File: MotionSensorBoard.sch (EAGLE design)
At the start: 21 parts, among them J1 PRGM, J2 POWER_JACKPTH, U1 ATTINY2313A-SUR, U2 ISO7221ADR, U4 NCP1117ST50T3G, U5 LM1117MPX-3.3

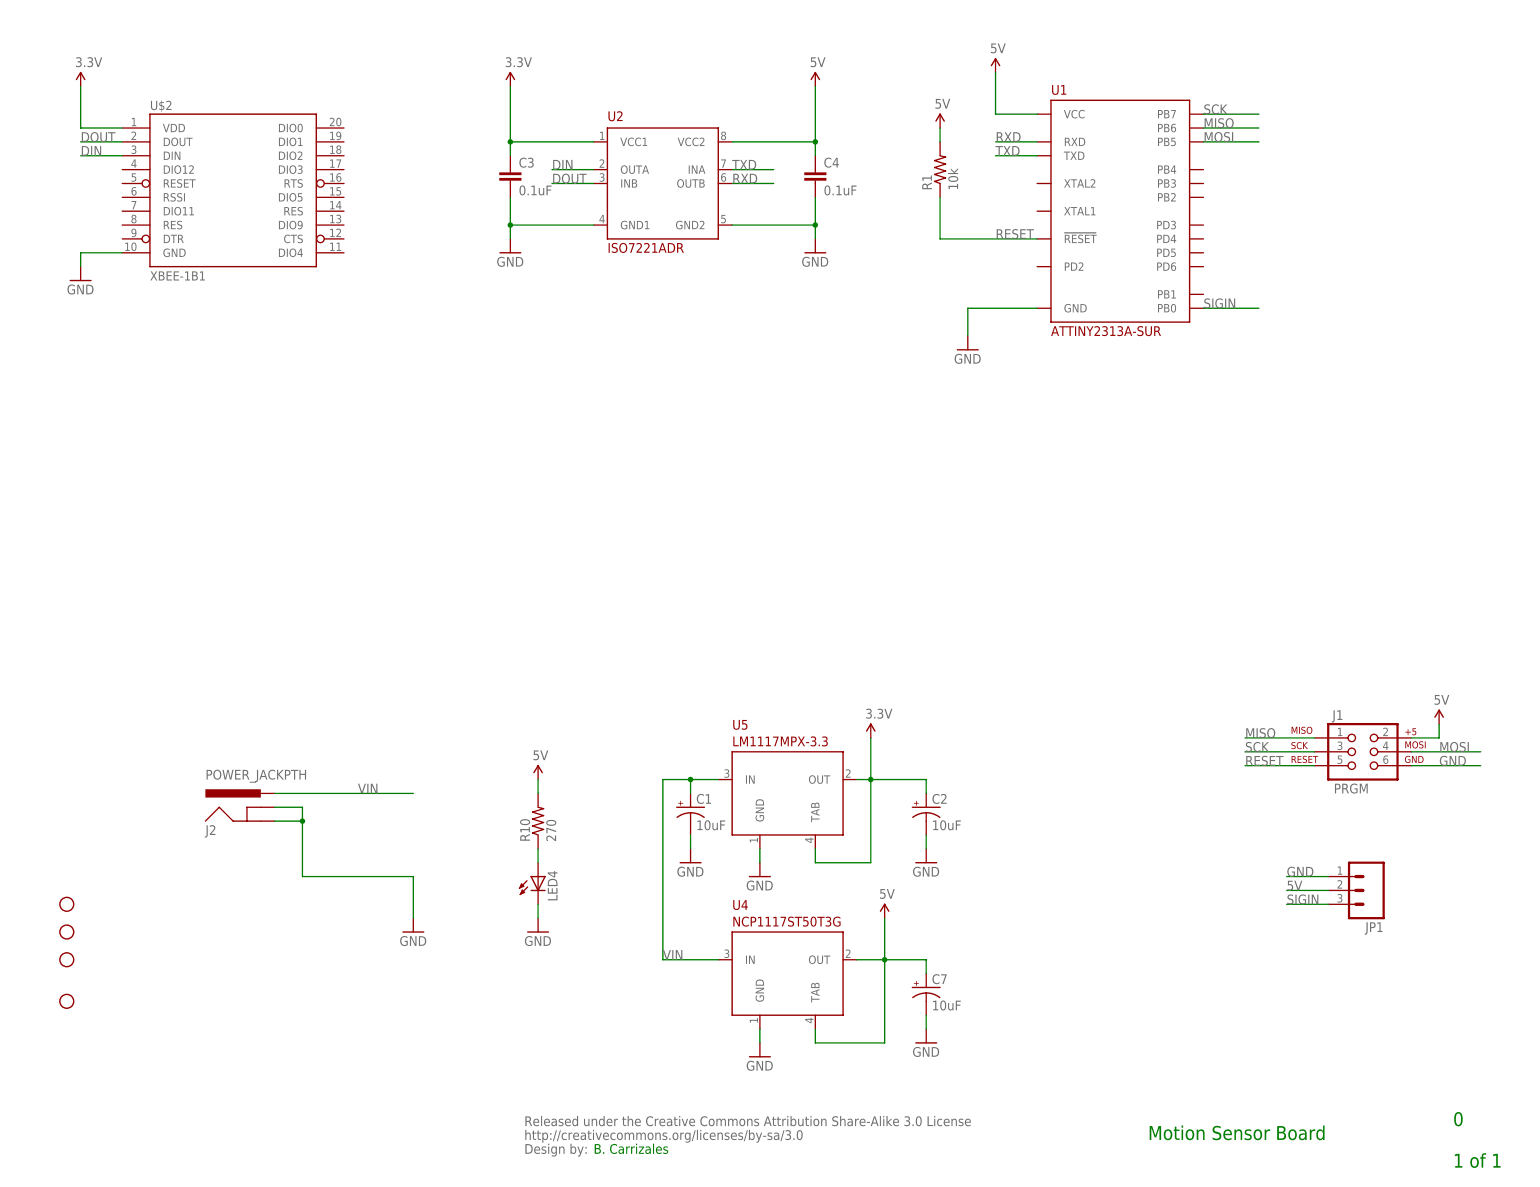
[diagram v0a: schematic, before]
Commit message: Schematic Updated
Schematic Rev A major revisions complete
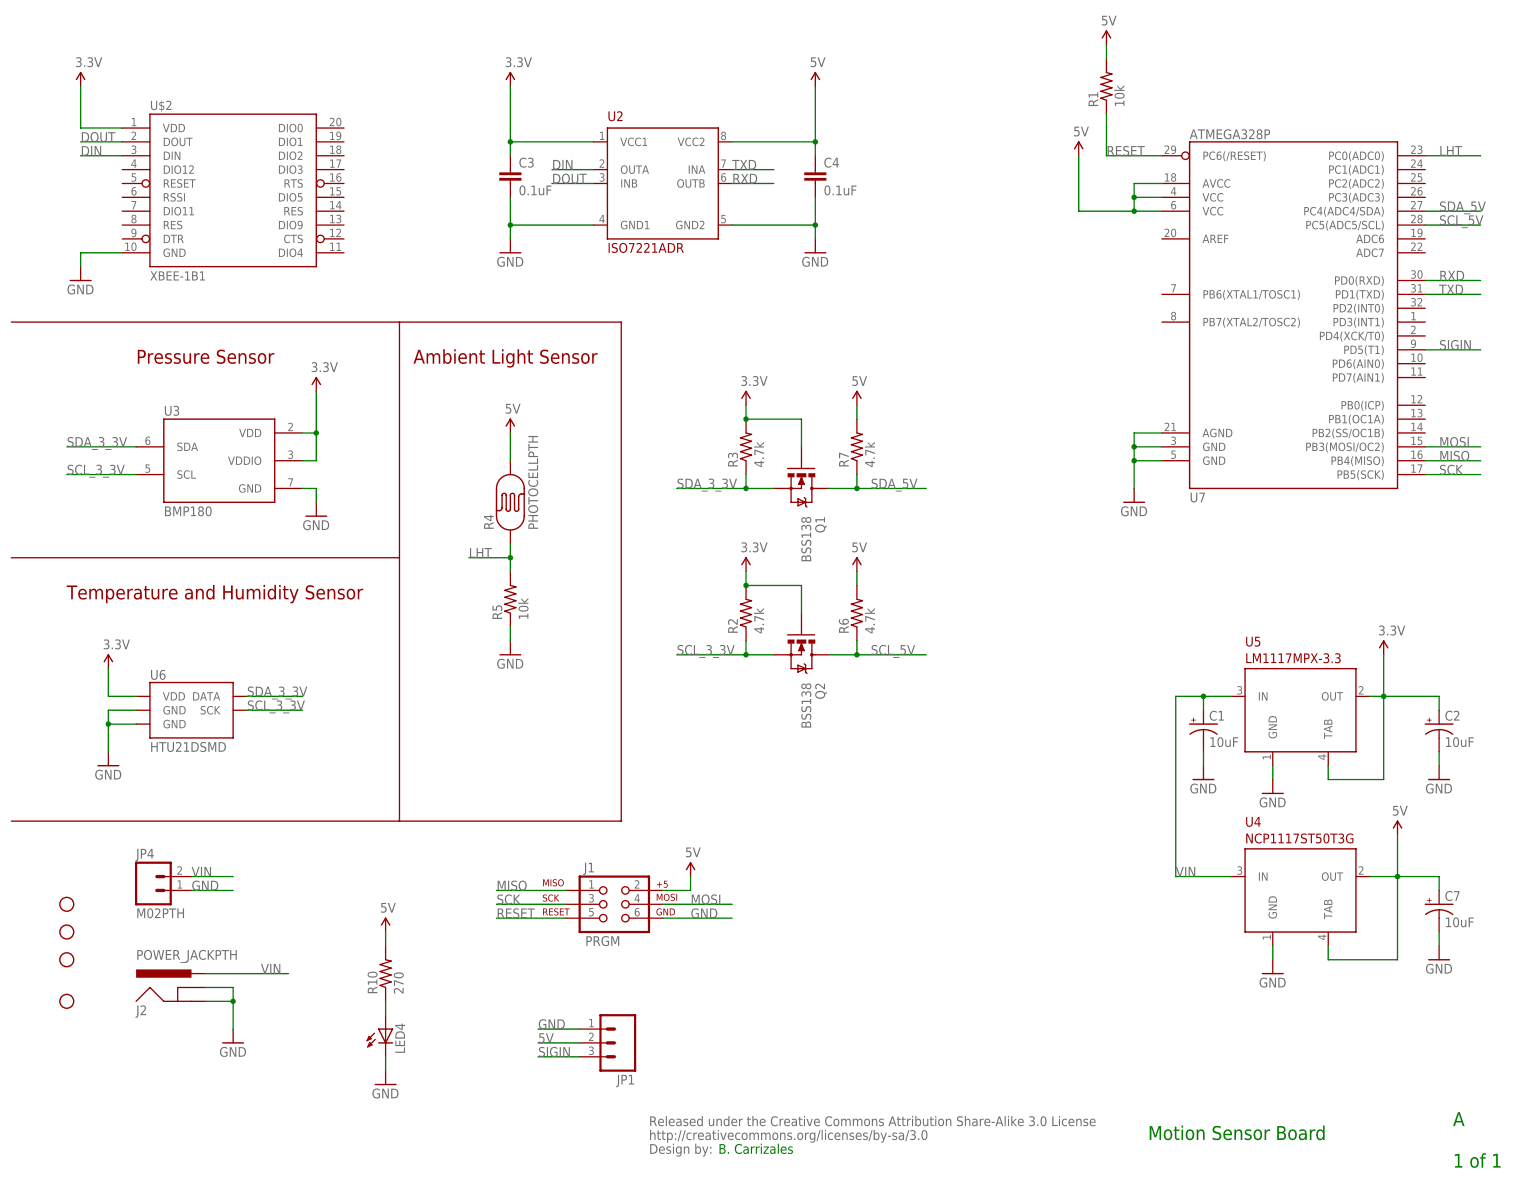
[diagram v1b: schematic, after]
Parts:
- removed U1: ATTINY2313A-SUR, microcontrollers-atmel:ATTINY2313A-SUR
- added JP4: M02PTH, SparkFun-Connectors:M02PTH
- added Q1, Q2: BSS138, SparkFun-DiscreteSemi:MOSFET-NCHANNELBSS123LT1G
- added R2, R3, R6, R7: 4.7k, SparkFun-Resistors:RESISTOR0603
- added R4: PHOTOCELLPTH, SparkFun-Sensors:PHOTOCELLPTH
- added R5: 10k, SparkFun-Resistors:RESISTOR0603
- added U3: BMP180, SparkFun-Sensors:BMP180
- added U6: HTU21DSMD, SparkFun-Sensors:HTU21DSMD
- added U7: ATMEGA328P, SparkFun-DigitalIC:ATMEGA328_SMT
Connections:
- new net LHT: R4.P$1, R5.2, U7.PC0(ADC0)
- new net SCL_3_3V: Q2.S, R2.1, U3.SCL, U6.SCK
- new net SCL_5V: Q2.D, R6.1, U7.PC5(ADC5/SCL)
- new net SDA_3_3V: Q1.S, R3.1, U3.SDA, U6.DATA
- new net SDA_5V: Q1.D, R7.1, U7.PC4(ADC4/SDA)
- net 3.3V: now also Q1.G, Q2.G, R2.2, R3.2, U3.VDD, U3.VDDIO, U6.VDD
- net 5V: now also R4.P$2, R6.2, R7.2, U7.AVCC, U7.VCC@1, U7.VCC@2; no longer U1.VCC
- net GND: now also JP4.1, R5.1, U3.GND, U6.GND@2, U6.GND@7, U7.AGND, U7.GND@1, U7.GND@2; no longer U1.GND
- net MISO: now also U7.PB4(MISO); no longer U1.PB6
- net MOSI: now also U7.PB3(MOSI/OC2); no longer U1.PB5
- net RESET: now also U7.PC6(/RESET); no longer U1.!RESET
- net RXD: now also U7.PD0(RXD); no longer U1.RXD
- net SCK: now also U7.PB5(SCK); no longer U1.PB7
- net SIGIN: now also U7.PD5(T1); no longer U1.PB0
- net TXD: now also U7.PD1(TXD); no longer U1.TXD
- net VIN: now also JP4.2
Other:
- note added: "A"
- note added: "Ambient Light Sensor"
- note added: "Pressure Sensor"
- note added: "Temperature and Humidity Sensor"
- note removed: "0"
- moved on the sheet: C1, C2, C7, J1, J2, JP1, LED4, R1, R10, U4, U5
